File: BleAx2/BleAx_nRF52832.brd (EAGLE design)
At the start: 30 x 20.1 mm, 42 parts, among them CN1 6p-2.54, J1 2.0MM-90D, U1 NRF52832, U2 MCP73832T-2ACI/OT-SOT23-5, U4 MIC5225-3.3, X1 FA-128, X2 32.768kHz

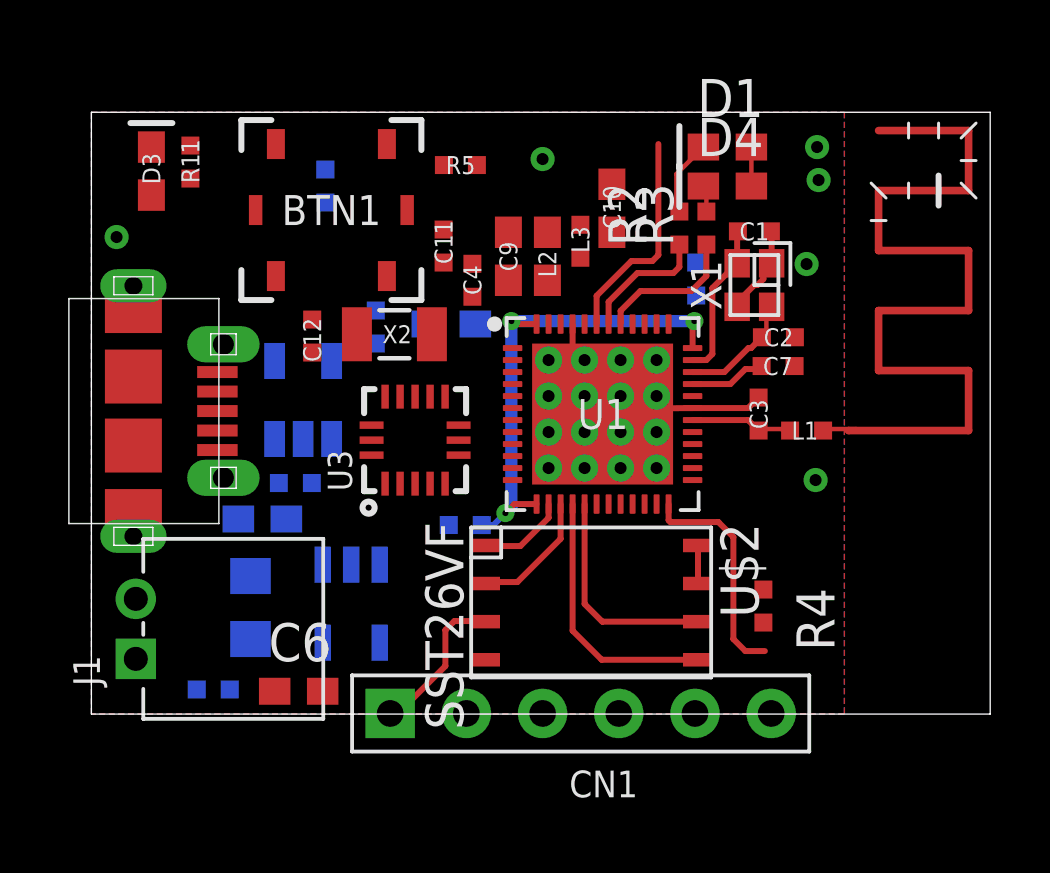
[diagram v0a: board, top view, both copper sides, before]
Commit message: evolve
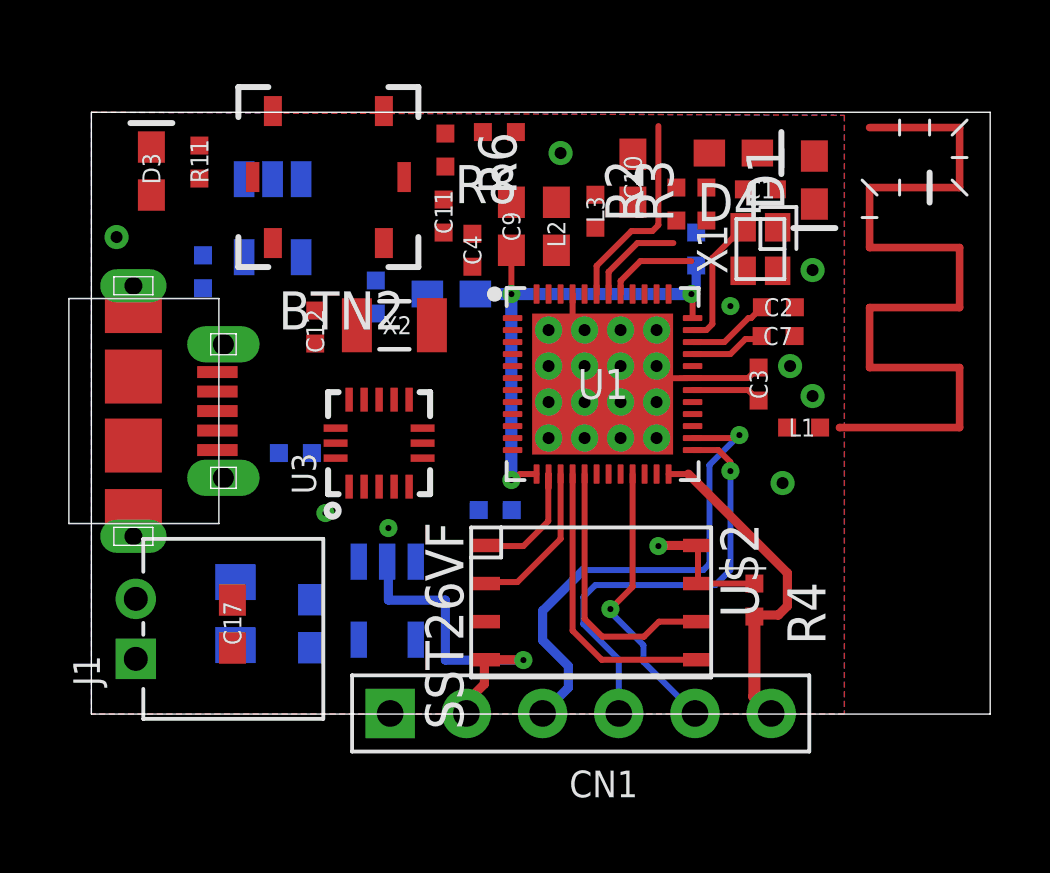
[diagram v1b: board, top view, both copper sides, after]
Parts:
- removed BTN1: PANASONIC_EVQPT5A15, Nordic_misc:PANASONIC_EVQPT5A15
- removed R5: 330R, Nordic_misc:RESC0402_N
- removed R7: 100k, Nordic_misc:RESC0402_N
- added BTN2: PANASONIC_EVQPT5A15, Nordic_misc:PANASONIC_EVQPT5A15
- added R6: 100k, Nordic_misc:RESC0402_N
- added R8: 330R, Nordic_misc:RESC0402_N
- moved R1 13.9 mm to (3.72, 14.7), turned to 270 degrees
- moved U2 6.15 mm to (6.04, 16.5), turned to 180 degrees
- moved C17 3.64 mm to (4.70, 3.00), flipped to the top, turned to 90 degrees
- moved D1 3.10 mm to (24.1, 17.8), turned to 90 degrees
- moved C6 2.29 mm to (7.34, 3.01), flipped to the bottom, turned to 90 degrees
- moved C1 1.41 mm to (22.3, 17.5)
- moved C10 1.22 mm to (18.1, 17.9)
- moved X1 1.22 mm to (22.3, 15.5)
- moved U3 1.20 mm to (9.59, 9.03)
- moved U4 1.20 mm to (9.86, 3.78)
- moved L3 1.12 mm to (16.8, 16.8)
- moved C5 1.12 mm to (13.5, 6.80)
- moved D4 1.12 mm to (21.4, 18.7), turned to 180 degrees
- moved L2 1.04 mm to (15.5, 16.3)
- moved C9 1.00 mm to (14.0, 16.3)
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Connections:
- removed net N$11: D1.1, R2.2
- removed net N$12: D4.1, R3.2
- removed net VCC: R4.1
- new net N$6: BTN2.1, BTN2.2, R6.1, R8.2
- new net N$8: D4.2, R3.2
- net BTTN_01: now also R8.1; no longer R5.1
- net GND: now also BTN2.3, BTN2.4, BTN2.5, BTN2.6, D1.1, D4.1; no longer BTN1.3, BTN1.4, BTN1.5, BTN1.6
- net N$7: now also D1.2, R2.2; no longer BTN1.1, BTN1.2, R5.2, R7.1
- net VDD_P3V3: now also R4.1, R6.2; no longer D1.2, D4.2, R7.2
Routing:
- net SWDIO: track 0.00 -> 18.6 mm, vias 0 -> 1
- net SWDCLK: track 0.00 -> 14.7 mm, vias 0 -> 1
- net P0.18/SWO: track 0.00 -> 9.45 mm, vias 0 -> 1
- net GND: track 27.0 -> 35.1 mm, vias 6 -> 9
- net P0.21/RESET: track 8.05 -> 11.1 mm
- net N$11: track 2.54 -> 0.00 mm, vias 0 -> 1
- net VDD_P3V3: track 24.2 -> 22.3 mm, vias 3 -> 4
- net LED_02: track 4.83 -> 3.07 mm
- net SCK_02: track 7.35 -> 9.06 mm
- net SST26_CE: track 2.98 -> 4.50 mm
- net N$5: track 1.39 -> 0.00 mm
- net ANT: track 3.40 -> 2.34 mm
- net LED_01: track 4.33 -> 3.30 mm
- net MOSI_02: track 8.80 -> 9.80 mm
- net MISO_02: track 4.30 -> 5.30 mm
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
